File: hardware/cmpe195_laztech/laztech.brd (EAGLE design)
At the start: 68.6 x 61 mm, 28 parts

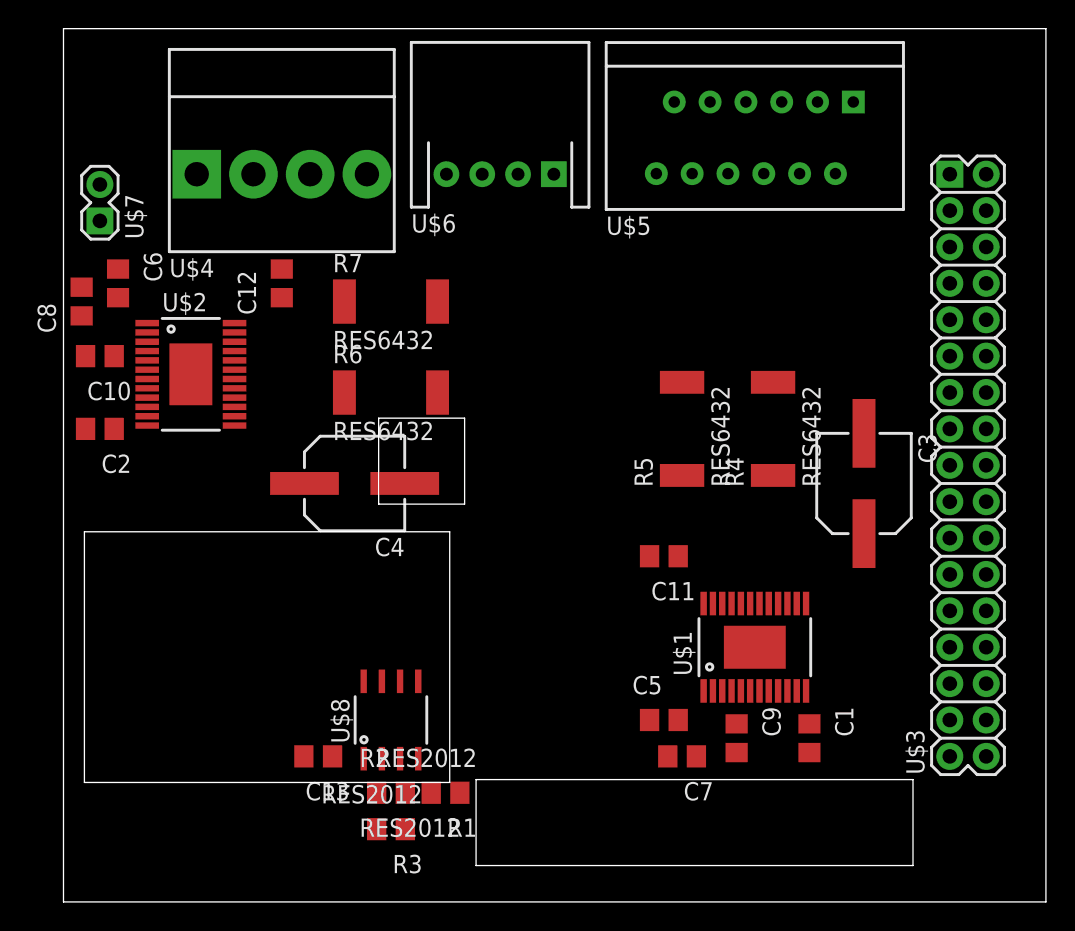
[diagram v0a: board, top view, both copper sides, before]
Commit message: Pre-route checkpoint.
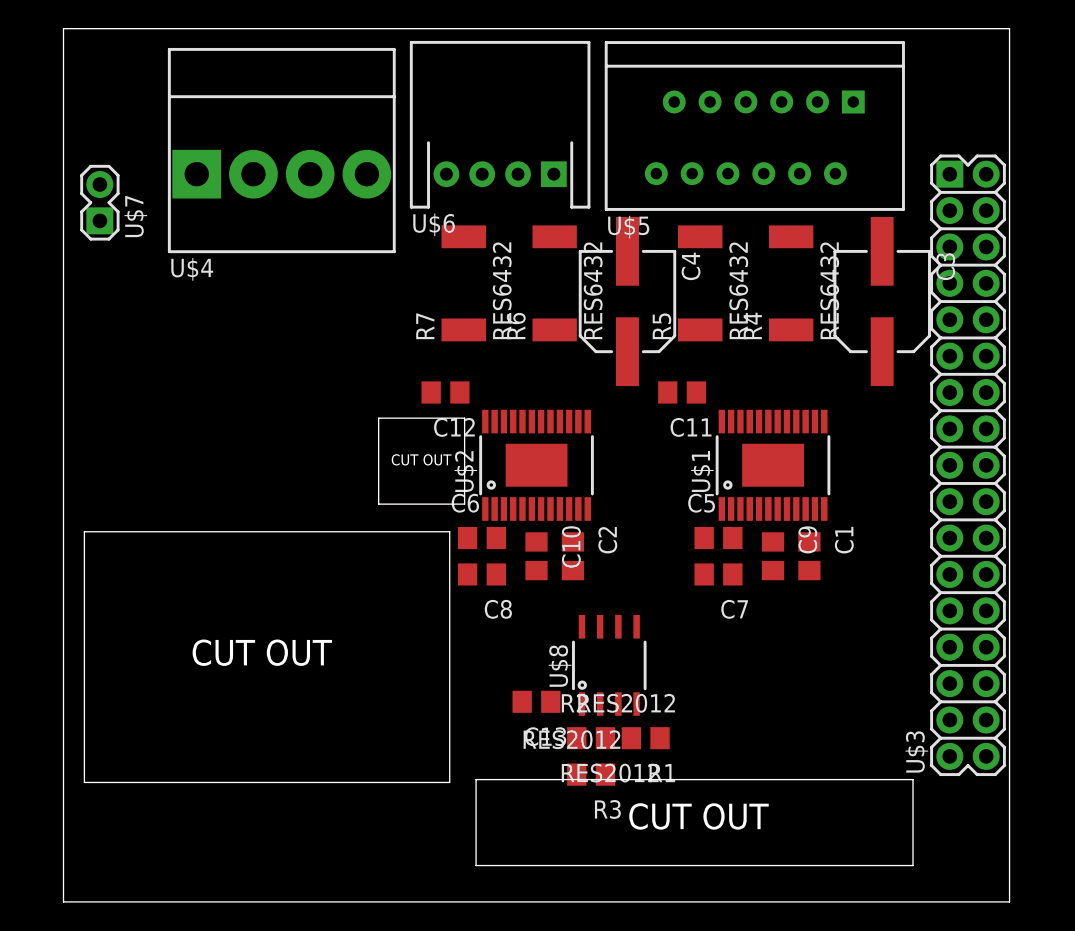
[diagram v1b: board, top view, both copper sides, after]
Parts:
- moved C2 34.2 mm to (35.6, 24.1), turned to 270 degrees
- moved C8 33.8 mm to (29.2, 22.9), turned to 180 degrees
- moved C10 33.5 mm to (33.0, 24.1), turned to 270 degrees
- moved C6 31.0 mm to (29.2, 25.4), turned to 0 degrees
- moved U$2 25.0 mm to (33.0, 30.5), turned to 0 degrees
- moved C4 22.9 mm to (39.4, 41.9), turned to 270 degrees
- moved C13 15.7 mm to (33.0, 14.0)
- moved U$8 15.7 mm to (38.1, 16.5)
- moved R1 14.5 mm to (40.6, 11.4)
- moved R2 14.5 mm to (36.8, 11.4)
- moved R3 14.5 mm to (36.8, 8.89)
- moved C12 13.7 mm to (26.7, 35.6), turned to 180 degrees
- moved R6 13.7 mm to (34.3, 43.2), turned to 90 degrees
- moved C5 13.3 mm to (45.7, 25.4)
- moved C7 13.0 mm to (45.7, 22.9)
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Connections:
- net N$1: now also U$5.10; no longer U$5.9
- net N$2: now also U$5.9; no longer U$5.10
- net N$5: now also U$2.15; no longer U$2.18
- net N$6: now also U$2.18; no longer U$2.15
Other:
- board size 68.6 x 61 mm -> 66 x 61 mm
- board text added: "CUT OUT"
